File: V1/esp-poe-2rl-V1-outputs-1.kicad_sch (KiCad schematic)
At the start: 80 parts, among them Q10 MMBT2222A/SOT-23-3, Q11 MMBT2222A/SOT-23-3, Q12 MMBT2222A/SOT-23-3, Q13 MMBT2222A/SOT-23-3, Q14 MMBT2222A/SOT-23-3, Q15 MMBT2222A/SOT-23-3, Q16 MMBT2222A/SOT-23-3, Q17 MMBT2222A/SOT-23-3, Q18 MMBT2222A/SOT-23-3, Q19 MMBT2222A/SOT-23-3, Q4 MMBT2222A/SOT-23-3, Q5 MMBT2222A/SOT-23-3, Q6 MMBT2222A/SOT-23-3, Q7 MMBT2222A/SOT-23-3, Q8 MMBT2222A/SOT-23-3, Q9 MMBT2222A/SOT-23-3

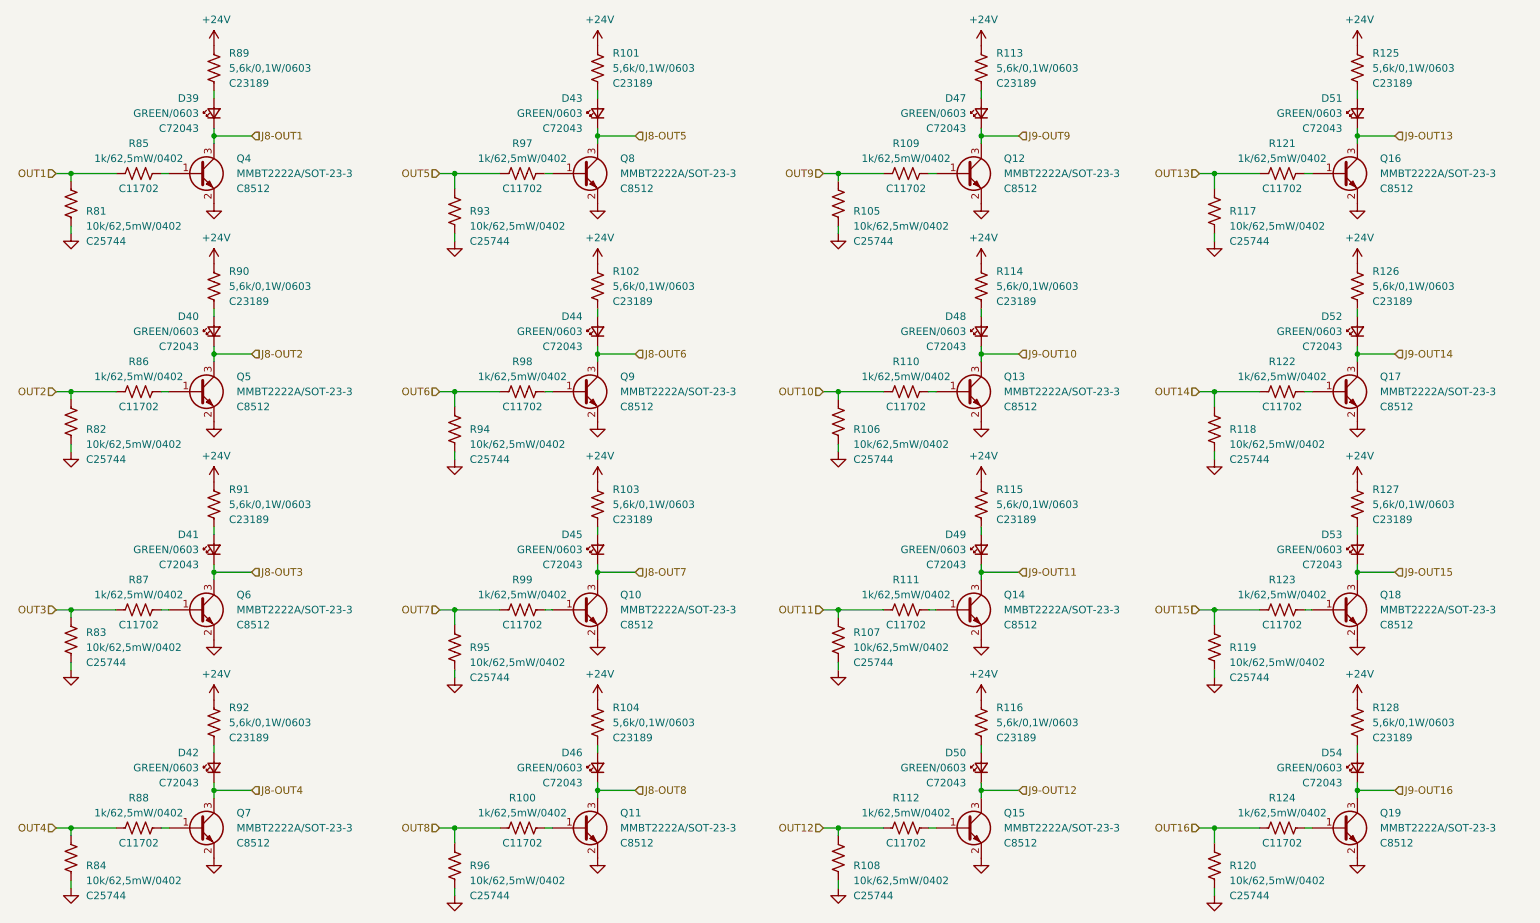
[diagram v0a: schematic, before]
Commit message: Dev
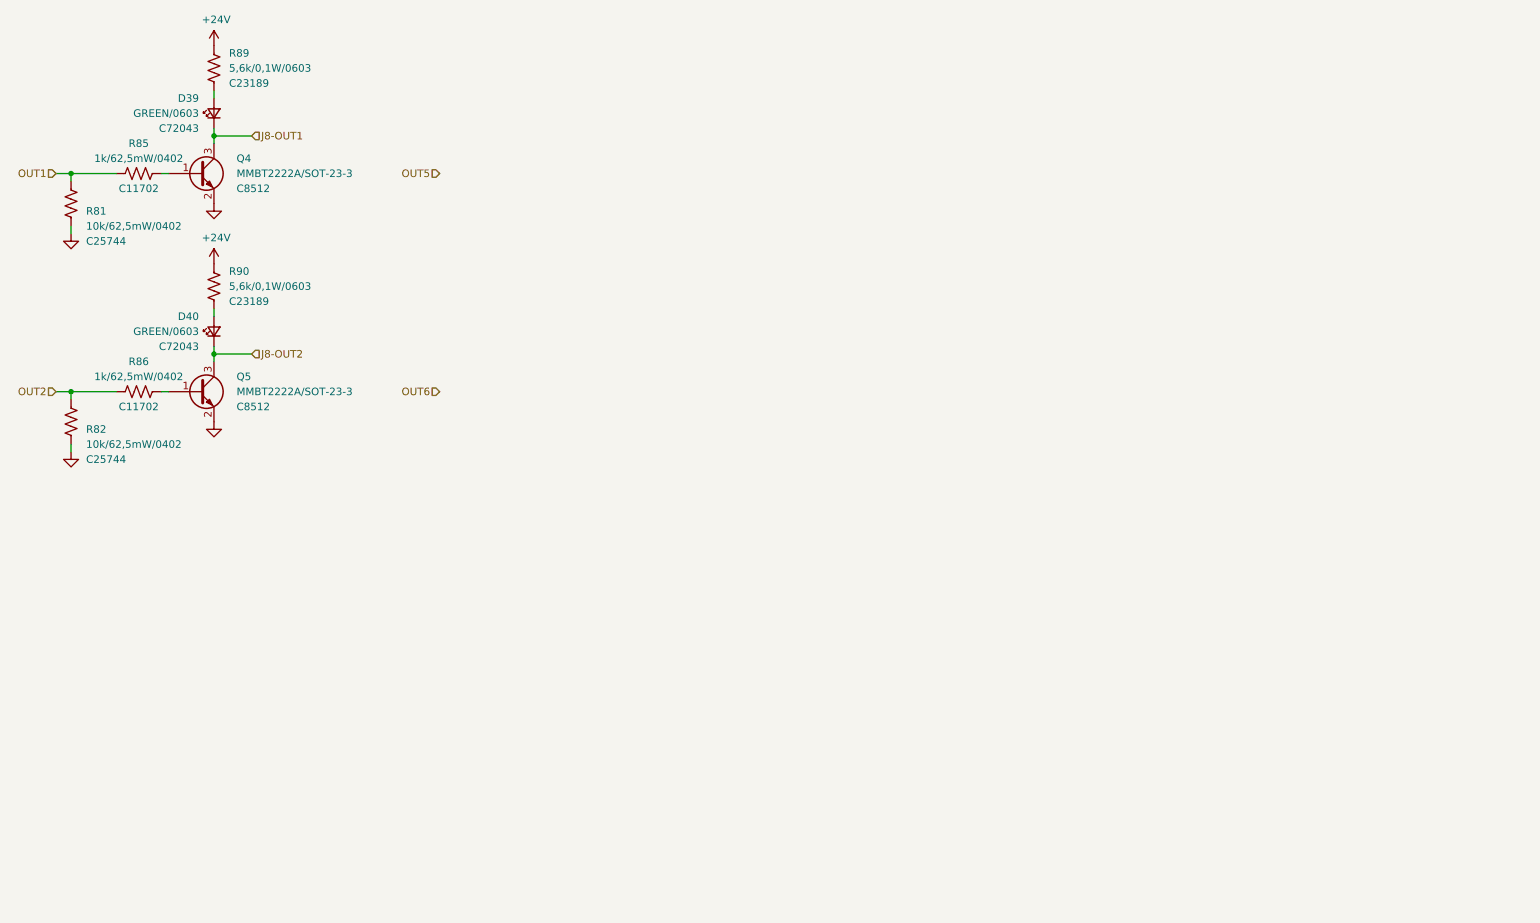
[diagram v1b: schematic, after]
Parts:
- removed D41, D42, D43, D44, D45, D46, D47, D48, D49, D50, D51, D52, D53, D54: GREEN/0603, Tales:LED_0603_1608Metric, symbol Device:LED_Small
- removed Q10, Q11, Q12, Q13, Q14, Q15, Q16, Q17, Q18, Q19, Q6, Q7, Q8, Q9: MMBT2222A/SOT-23-3, Tales:SOT-23, symbol Device:Q_NPN_BEC
- removed R100, R109, R110, R111, R112, R121, R122, R123, R124, R87, R88, R97, R98, R99: 1k/62,5mW/0402, Tales:R_0402_1005Metric, symbol Device:R_US
- removed R101, R102, R103, R104, R113, R114, R115, R116, R125, R126, R127, R128, R91, R92: 5,6k/0,1W/0603, Tales:R_0603_1608Metric, symbol Device:R_US
- removed R105, R106, R107, R108, R117, R118, R119, R120, R83, R84, R93, R94, R95, R96: 10k/62,5mW/0402, Tales:R_0402_1005Metric, symbol Device:R_US
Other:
- title: ESP 16x 24VDC Input 16x 24VDC Output Module -> ESP 2x Relay Output Module with PoE
